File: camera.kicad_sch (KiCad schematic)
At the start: 49 parts, among them J3 Conn_Coaxial, J4 Conn_01x06_Pin, J5 Conn_01x06_Pin, J6 Conn_01x06_Pin, J7 Conn_01x06_Pin, U6 SE5005L, U7 RTC6705, U8 HEF4051BT, Y2 8MHz

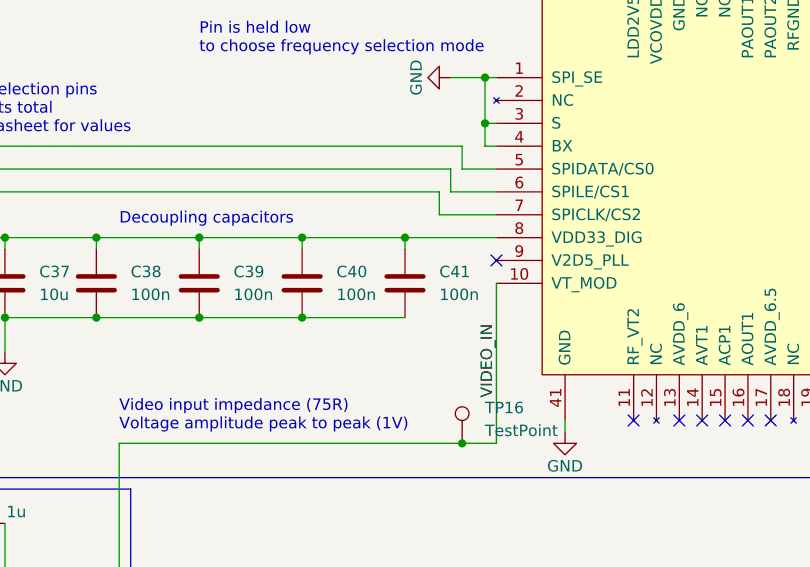
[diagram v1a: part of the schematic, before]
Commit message: Some routing
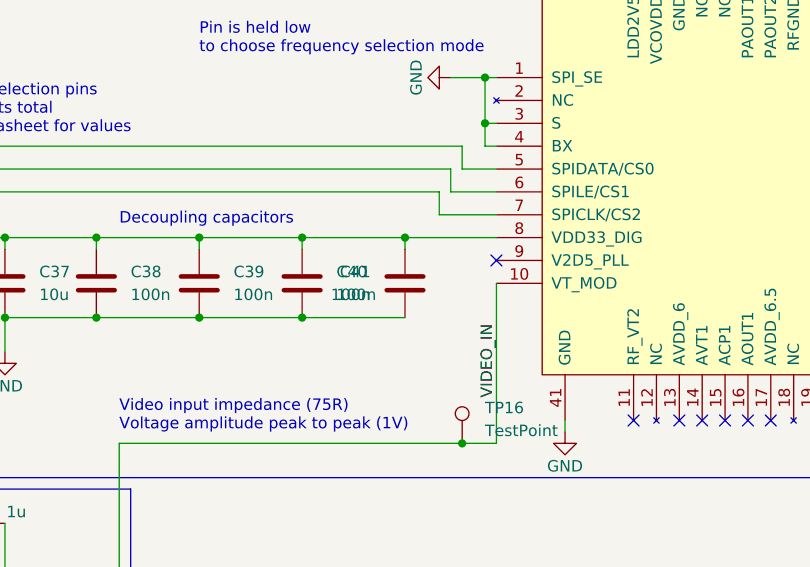
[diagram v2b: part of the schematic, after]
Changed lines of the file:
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@@
     )
   )
-  (symbol (lib_id "Device:C") (at 161.29 138.43 0) (unit 1)
-    (in_bom yes) (on_board yes) (dnp no) (fields_autoplaced)
-    (property "Reference" "C41" (at 165.1 137.1599 0)
+  (symbol (lib_id "Device:C") (at 161.29 138.43 0) (mirror y) (unit 1)
+    (in_bom yes) (on_board yes) (dnp no)
+    (property "Reference" "C41" (at 157.48 137.1599 0)
       (effects (font (size 1.27 1.27)) (justify left))
     )
-    (property "Value" "100n" (at 165.1 139.6999 0)
+    (property "Value" "100n" (at 157.48 139.6999 0)
       (effects (font (size 1.27 1.27)) (justify left))
     )
-    (property "Footprint" "Capacitor_SMD:C_0402_1005Metric" (at 162.2552 142.24 0)
+    (property "Footprint" "Capacitor_SMD:C_0402_1005Metric" (at 160.3248 142.24 0)
       (effects (font (size 1.27 1.27)) hide)
     )
